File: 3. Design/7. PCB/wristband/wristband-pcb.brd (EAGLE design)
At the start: 27.5 x 39.4 mm, 45 parts, among them IC1 STM32F051K8T6, Y2 FA-20H_16.0000MF12Z-AC3, Y3 FA-20H_16.0000MF12Z-AC3

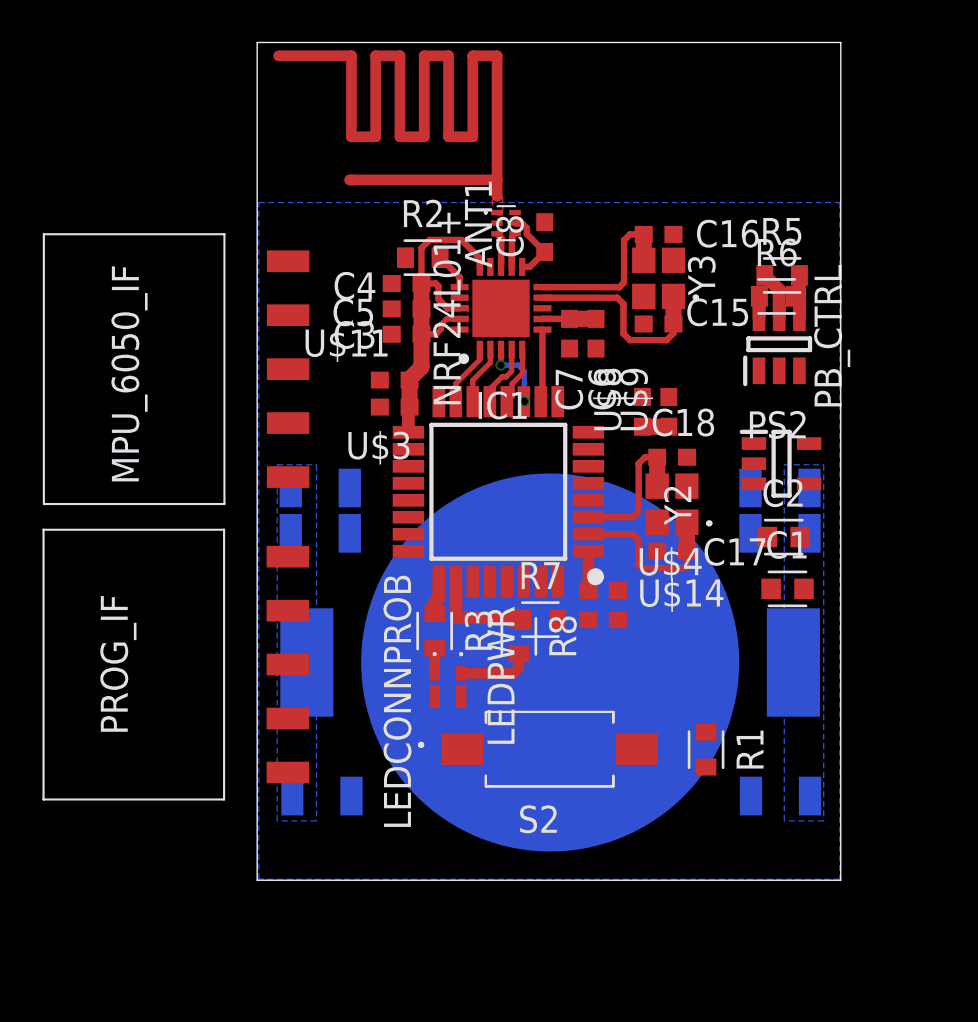
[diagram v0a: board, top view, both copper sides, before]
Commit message: UPDT: Wristband PCB
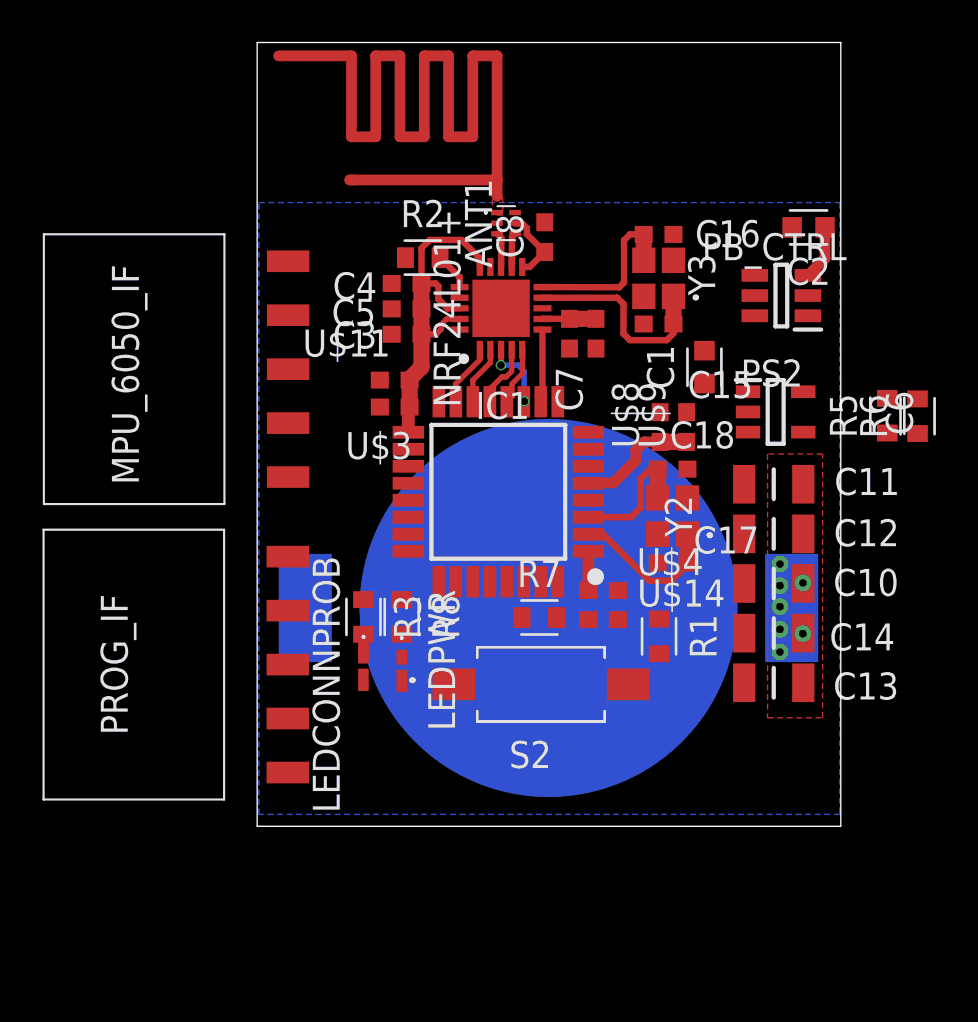
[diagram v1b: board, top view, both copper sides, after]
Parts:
- removed C9: 22nF [1206], CL31B226KPHNNNE:CAPC3216X180N
- moved C13 22.5 mm to (24.3, 9.30), flipped to the top
- moved C14 22.4 mm to (24.3, 11.6), flipped to the top
- moved C2 14.6 mm to (26.0, 30.7), turned to 180 degrees
- moved C1 11.1 mm to (21.1, 24.2), turned to 90 degrees
- moved C10 10.0 mm to (24.3, 14.0), flipped to the top, turned to 180 degrees
- moved R6 8.70 mm to (31.1, 21.8), turned to 90 degrees
- moved R5 8.26 mm to (29.7, 21.9), turned to 90 degrees
- moved R1 5.77 mm to (18.9, 11.5)
- moved R8 5.59 mm to (6.81, 12.4)
- moved LEDCONNPROB 3.45 mm to (5.00, 9.91)
- moved R3 3.42 mm to (5.00, 12.4)
- moved S2 3.07 mm to (13.4, 9.22)
- moved LEDPWR 2.90 mm to (6.81, 9.86)
- moved BATT_HLD 2.57 mm to (13.7, 12.8)
- moved PS2 2.45 mm to (24.4, 22.0)
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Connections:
- new net S$1: R5.1
- net GND: no longer C9.2
- net PWR_CLR: no longer IC1.6, R6.1
- net PWR_INT: no longer IC1.7, R5.1
- net VCC_BATT: no longer C9.1
- net VDD: no longer PS2.1
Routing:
- net LED_PWR: track 4.72 -> 0.00 mm
- net VDDA: track 1.24 -> 5.71 mm
- net N$6: track 3.49 -> 0.00 mm
- net N$5: track 3.21 -> 0.00 mm
- net VCC_BATT: track 0.00 -> 2.59 mm, vias 0 -> 6
- net PWR_INT: track 2.27 -> 0.00 mm
- net LED_CONN_PROB: track 1.60 -> 0.04 mm
- net PWR_CLR: track 1.01 -> 0.00 mm
- net STM32F051_CRYSTAL1: track 8.06 -> 7.32 mm
- net STM32F051_CRYSTAL2: track 7.08 -> 6.43 mm
- added copper zone on layer 1, net VCC_BATT
- removed copper zone on layer 1, net GND
- removed copper zone on layer 16, net VCC_BATT
- removed copper zone on layer 1, net VDD
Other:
- board size 27.5 x 39.4 mm -> 27.5 x 36.9 mm

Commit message: UPDT: Further updates to the wristband PCB
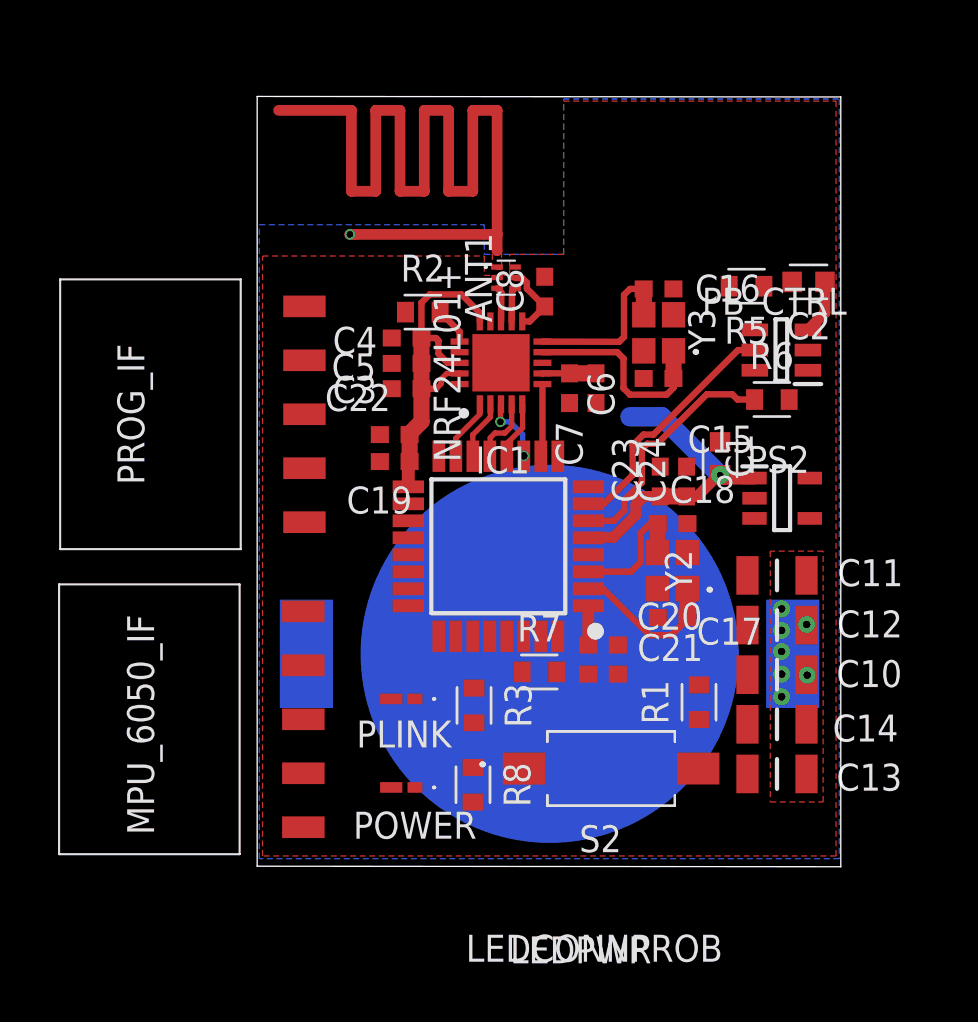
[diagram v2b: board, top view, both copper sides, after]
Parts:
- removed U$11, U$14, U$9: 10nF [0603], Nordic_nRF:RESC0603_L
- removed U$2: MIFA-CYPRESS-2, MIFA:MIFA-CYPRESS-2
- removed U$3, U$4: 4.7uF [0603], Nordic_nRF:RESC0603_L
- removed U$8: 1uF [0603], Nordic_nRF:RESC0603_L
- added C19, C20: 4.7uF [0603], Nordic_nRF:RESC0603_L
- added C21, C22, C24: 10nF [0603], Nordic_nRF:RESC0603_L
- added C23: 1uF [0603], Nordic_nRF:RESC0603_L
- added MIFA: MIFA-CYPRESS-2, MIFA:MIFA-CYPRESS-2
- moved MPU_6050_IF 16.5 mm to (-3.08, 7.58)
- moved PROG_IF 11.8 mm to (-3.02, 21.9)
- moved R5 9.01 mm to (23.0, 28.0), turned to 180 degrees
- moved R8 8.58 mm to (10.2, 4.50)
- moved R6 6.90 mm to (24.2, 22.6), turned to 0 degrees
- moved R3 6.67 mm to (10.2, 8.23)
- moved LEDPWR 5.49 mm to (6.78, 4.37), turned to 180 degrees
- moved S2 5.16 mm to (16.7, 5.26)
- moved C1 4.36 mm to (21.8, 19.9)
- moved C10 4.30 mm to (24.5, 9.68)
- moved C13 4.30 mm to (24.5, 5.00)
- moved C14 4.30 mm to (24.5, 7.34)
- moved C11 4.30 mm to (24.5, 14.4)
- moved C12 4.30 mm to (24.5, 12.0)
- moved PS2 4.08 mm to (24.7, 18.0)
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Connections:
- net N$5 renamed PWR_EN
- removed net N$1: ANT1.1, U$2.ANT
- removed net S$1: R5.1
- removed net VDDA: IC1.5, U$8.1, U$9.1
- new net MIFA: ANT1.1, MIFA.ANT
- net GND: now also C19.2, C20.2, C21.2, C22.2, C23.2, C24.2, MIFA.GND; no longer U$11.2, U$14.2, U$2.GND, U$3.2, U$4.2, U$8.2, U$9.2
- net PWR_CLR: now also IC1.6, R6.1
- net PWR_INT: now also IC1.7, R5.1
- net VDD: now also C19.1, C20.1, C21.1, C22.1, C23.1, C24.1, IC1.5, PS2.1; no longer U$11.1, U$14.1, U$3.1, U$4.1
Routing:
- net VDD: track 21.9 -> 36.7 mm, vias 0 -> 1
- net PWR_INT: track 0.00 -> 11.7 mm
- net PWR_CLR: track 0.00 -> 11.6 mm
- net VDDA: track 5.71 -> 0.00 mm
- net N$7: track 1.03 -> 0.00 mm
- added copper zone on layer 1, net GND
- added copper zone on layer 1, net MIFA
- removed copper zone on layer 1, net N$1
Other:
- board size 27.5 x 36.9 mm -> 27.5 x 36.3 mm
- board text added: "PLINK"
- board text added: "POWER"

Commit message: UPDT: Wristband PCB
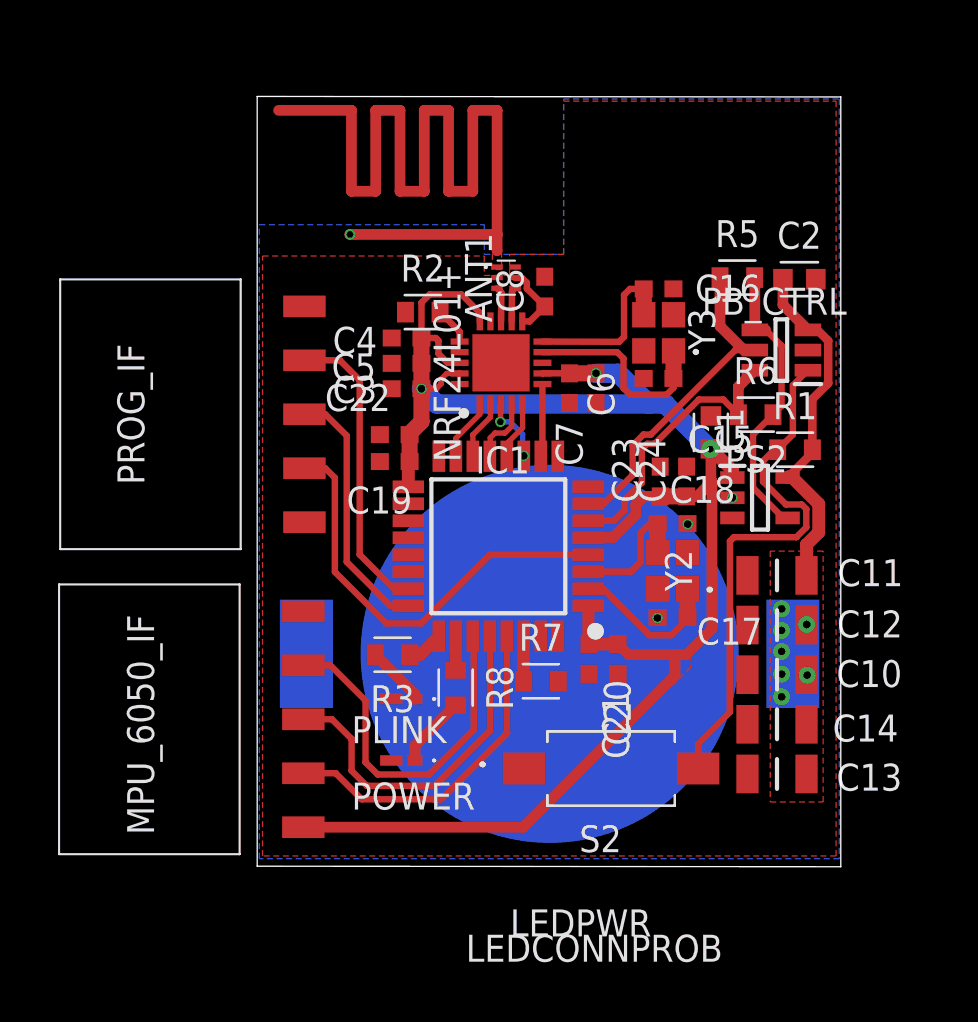
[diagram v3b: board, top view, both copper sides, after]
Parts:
- moved R1 12.7 mm to (25.3, 20.3), turned to 0 degrees
- moved R8 4.64 mm to (9.35, 9.07)
- moved R3 4.52 mm to (6.38, 10.6), turned to 180 degrees
- moved C1 1.29 mm to (21.4, 21.1)
- moved LEDPWR 1.27 mm to (6.78, 5.64)
- moved R6 1.04 mm to (23.5, 21.9)
- moved PS2 1.04 mm to (23.7, 18.0)
- moved C21 0.97 mm to (15.6, 10.4), turned to 270 degrees
- moved C20 0.97 mm to (17.0, 10.4), turned to 270 degrees
- moved R5 0.59 mm to (22.6, 28.4), turned to 0 degrees
- moved C2 0.45 mm to (25.5, 28.3), turned to 0 degrees
- moved R7 0.44 mm to (13.4, 9.37)
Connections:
- net GND: now also MPU_6050_IF.5; no longer MPU_6050_IF.4
- net MPU_6050_INT: now also MPU_6050_IF.4; no longer MPU_6050_IF.5
- net MPU_6050_SCL: now also MPU_6050_IF.3; no longer MPU_6050_IF.2
- net MPU_6050_SDA: now also MPU_6050_IF.2; no longer MPU_6050_IF.3
- net SYS_NRST: now also PROG_IF.2; no longer PROG_IF.4
- net SYS_SWCLK: now also PROG_IF.3; no longer PROG_IF.2
- net SYS_SWDIO: now also PROG_IF.4; no longer PROG_IF.3
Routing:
- net VDD: track 36.7 -> 86.6 mm, vias 1 -> 3
- net N$2: track 0.00 -> 24.8 mm
- net SYS_NRST: track 0.00 -> 20.3 mm
- net MPU_6050_INT: track 0.00 -> 17.2 mm
- net MPU_6050_SCL: track 0.00 -> 16.5 mm
- net MPU_6050_SDA: track 0.00 -> 16.0 mm
- net VCC_BATT: track 2.59 -> 16.9 mm
- net SYS_SWDIO: track 0.00 -> 14.2 mm
- net PWR_EN: track 0.00 -> 13.7 mm
- net SYS_SWCLK: track 0.00 -> 12.1 mm
- net PWR_INT: track 11.7 -> 16.0 mm
- net N$6: track 0.00 -> 3.41 mm
- net N$7: track 0.00 -> 2.86 mm
- net N$4: track 0.00 -> 2.12 mm
- net PWR_CLR: track 11.6 -> 13.3 mm
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- added copper zone on layer 1, net VDD
